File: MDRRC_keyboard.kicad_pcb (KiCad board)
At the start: 2 copper layers, 43.6 x 21 mm, 21 parts, among them CON1 AVR-ISP-6, IC1 ATMEGA8-AI, P1 LCD, P2 CONN_8, P3 CONN_4, P4 CONN_4X2, X1 CRYSTAL

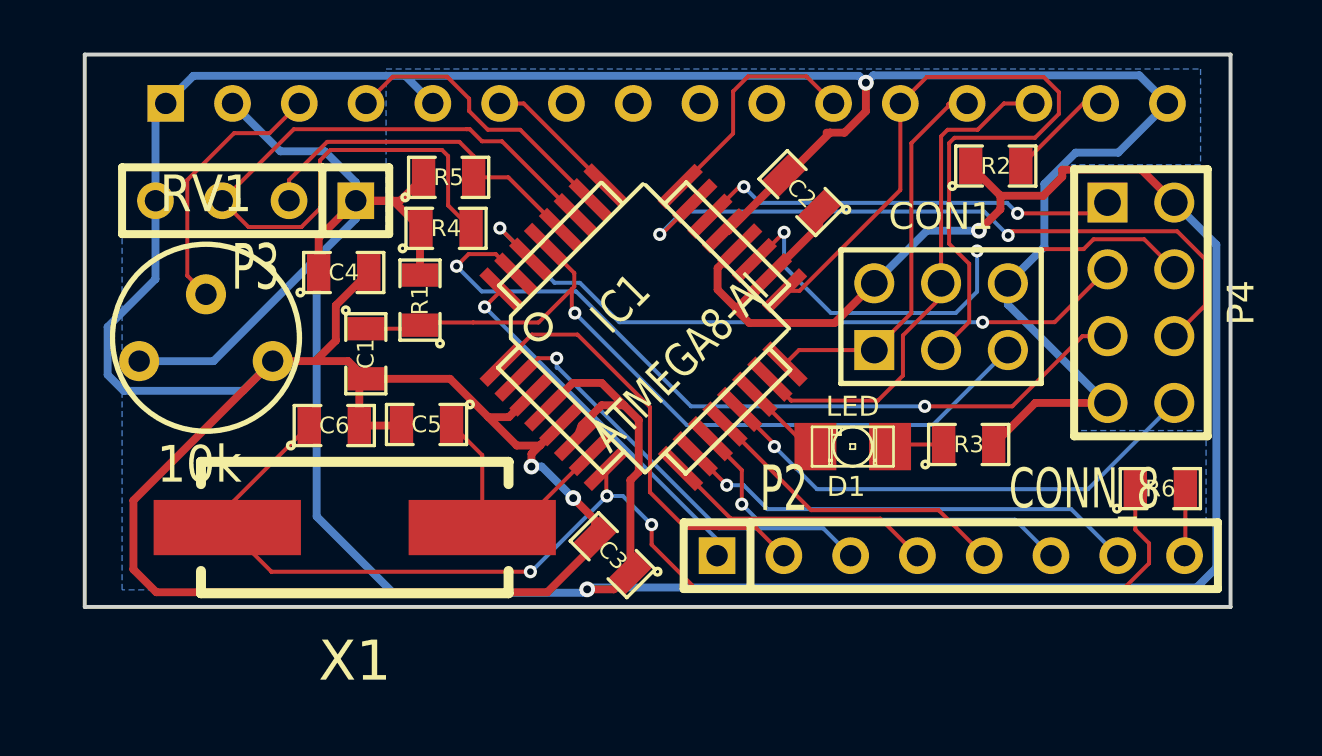
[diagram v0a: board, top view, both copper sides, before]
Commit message: Silkscreen update, rev 0
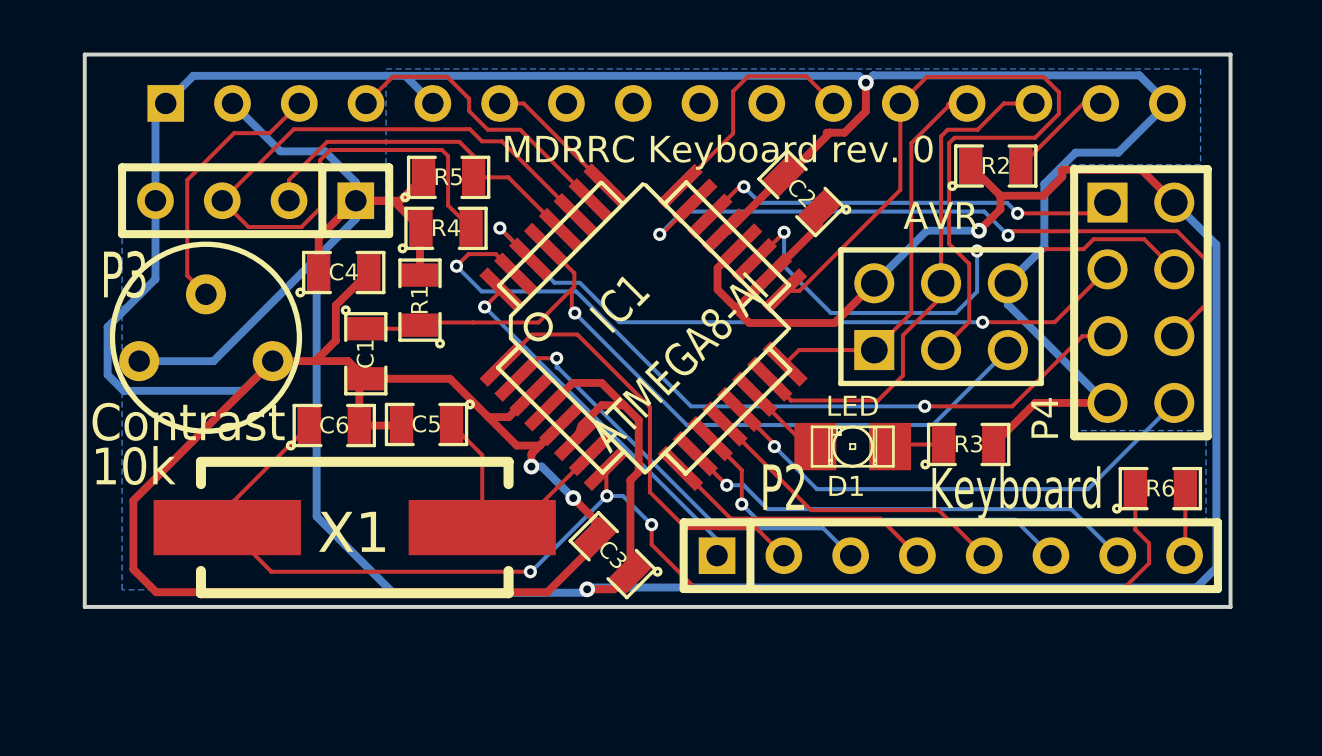
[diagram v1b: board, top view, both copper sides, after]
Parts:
- added ?: , dp_devices-CC-BY-SA, B.Cu at (154.9, 86.9)
- P2: value CONN_8 -> Keyboard
- renumbered CON1 to AVR, RV1 to Contrast
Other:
- board text added: "3. PD0 4. ADC6 5. PD1"
- board text added: "6. PC0 7. GND 8. PB1"
- board text added: "MDRRC Keyboard rev. 0"
- board text added: "Original schematic: Robert Everts Extended by, Board by: Dirkjan Krijnders"
- board text added: "P1: 1. Vcc 2. SCL 3. SDA 4. GND"
- board text added: "P4: 1. ADC7 2. Vcc"
- board text added: "https://github.com/dirkjankrijnders/MDRRC-Keyboard"
